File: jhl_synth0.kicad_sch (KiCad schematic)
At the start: 17 parts, among them J1 Conn_01x04, J2 USB_B_Micro, J3 Conn_01x04, J4 Conn_01x04, J5 Conn_01x01, J7 Conn_01x08, U1 YAAJ_BluePill, U2 YAAJ_BlackPill, U3 NUCLEO-F303K8

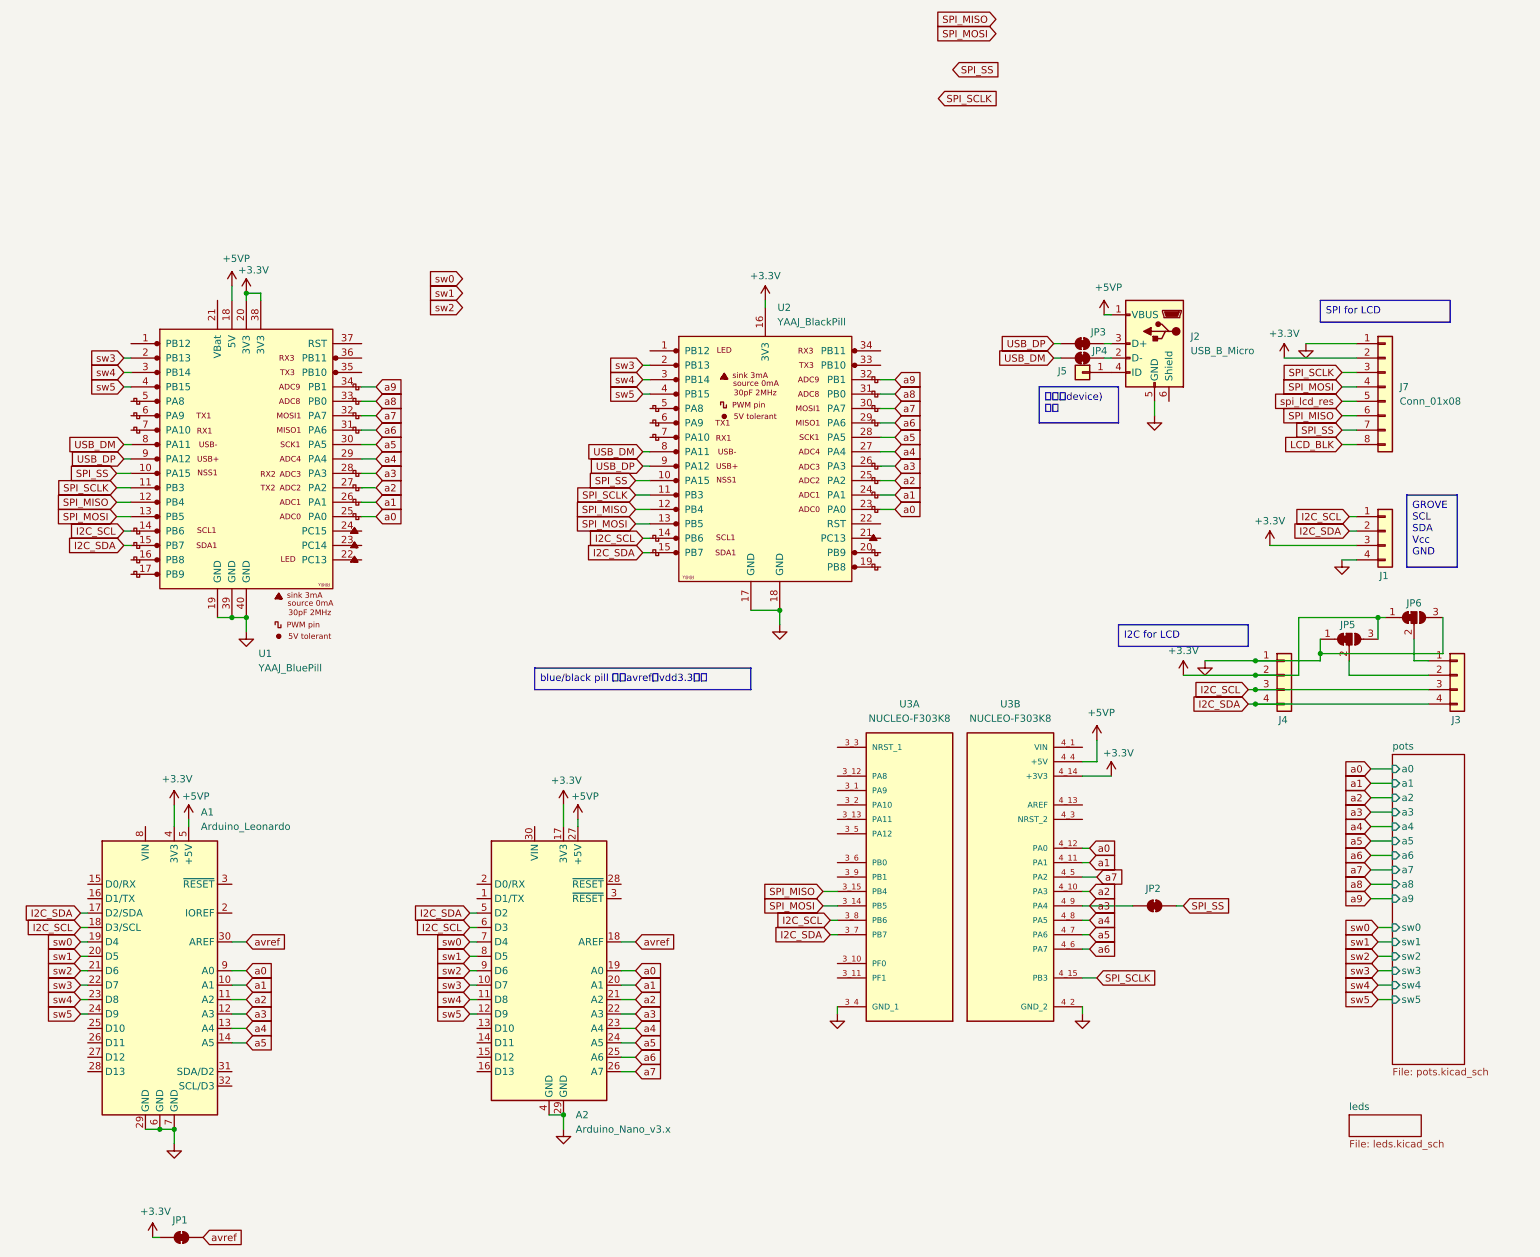
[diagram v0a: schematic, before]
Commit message: 251023
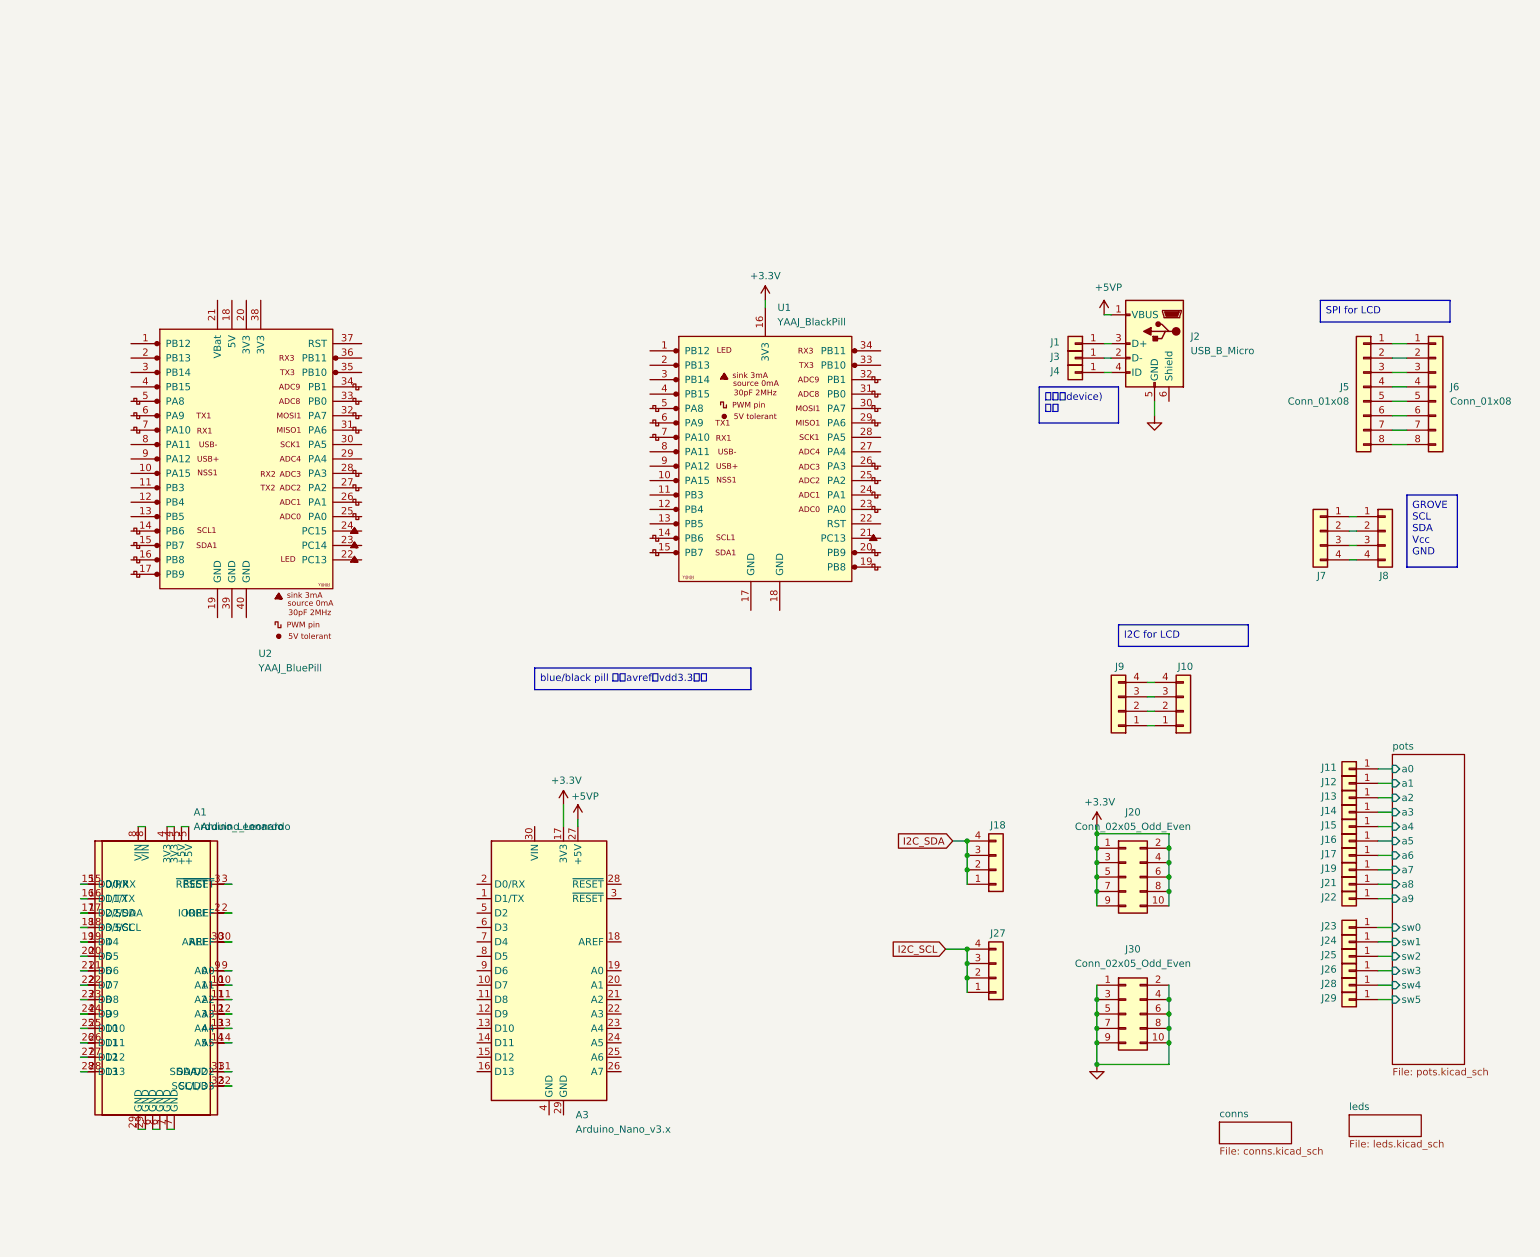
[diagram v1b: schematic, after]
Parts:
- removed J3, J4: Conn_01x04, Connector_PinSocket_2.54mm:PinSocket_1x04_P2.54mm_Vertical, symbol Connector_Generic:Conn_01x04
- removed JP1, JP2, JP3, JP4: SolderJumper_2_Bridged, Jumper:SolderJumper-2_P1.3mm_Bridged_RoundedPad1.0x1.5mm, symbol Jumper:SolderJumper_2_Bridged
- removed JP5, JP6: SolderJumper_3_Bridged12, Jumper:SolderJumper-3_P1.3mm_Bridged12_RoundedPad1.0x1.5mm, symbol Jumper:SolderJumper_3_Bridged12
- removed U3: NUCLEO-F303K8, NUCLEO-F303K8:MODULE_NUCLEO-F303K8, symbol NUCLEO-F303K8:NUCLEO-F303K8
- added A1: Arduino_Leonardo, Module:Arduino_UNO_R3, symbol MCU_Module:Arduino_Leonardo
- added J1, J11, J12, J13, J14, J15, J16, J17, J19, J21, J22, J23, J24, J25, J26, J28, J29, J3: Conn_01x01, Connector_PinSocket_2.54mm:PinSocket_1x01_P2.54mm_Vertical, symbol Connector_Generic:Conn_01x01
- added J10, J18, J27, J7, J9: Conn_01x04, Connector_PinSocket_2.54mm:PinSocket_1x04_P2.54mm_Vertical, symbol Connector_Generic:Conn_01x04
- added J20, J30: Conn_02x05_Odd_Even, Connector_PinHeader_2.54mm:PinHeader_2x05_P2.54mm_Vertical, symbol Connector_Generic:Conn_02x05_Odd_Even
- added J6: Conn_01x08, Connector_PinHeader_2.54mm:PinHeader_1x08_P2.54mm_Vertical, symbol Connector_Generic:Conn_01x08
- renumbered A1 to A2, A2 to A3, J5 to J4, J7 to J5, J1 to J8, U2 to U1, U1 to U2
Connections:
- net +3.3V: now also J20.1 (Pin_1), J20.10 (Pin_10), J20.2 (Pin_2), J20.3 (Pin_3), J20.4 (Pin_4), J20.5 (Pin_5), J20.6 (Pin_6), J20.7 (Pin_7), J20.8 (Pin_8), J20.9 (Pin_9); no longer A2.4 (3V3), J5.2 (Pin_2), J8.3 (Pin_3), U2.20 (3V3), U2.38 (3V3)
- net +5VP: no longer A2.5 (+5V), U2.18 (5V)
- net GND: now also J30.1 (Pin_1), J30.10 (Pin_10), J30.2 (Pin_2), J30.3 (Pin_3), J30.4 (Pin_4), J30.5 (Pin_5), J30.6 (Pin_6), J30.7 (Pin_7), J30.8 (Pin_8), J30.9 (Pin_9); no longer A2.29 (GND), A2.6 (GND), A2.7 (GND), A3.29 (GND), A3.4 (GND), J5.1 (Pin_1), J8.4 (Pin_4), U1.17 (GND), U1.18 (GND), U2.19 (GND), U2.39 (GND), U2.40 (GND)
- net I2C_SCL: now also J27.1 (Pin_1), J27.2 (Pin_2), J27.3 (Pin_3), J27.4 (Pin_4); no longer A2.18 (D3/SCL), A3.6 (D3), J8.1 (Pin_1), U1.14 (PB6), U2.14 (PB6)
- net I2C_SDA: now also J18.1 (Pin_1), J18.2 (Pin_2), J18.3 (Pin_3), J18.4 (Pin_4); no longer A2.17 (D2/SDA), A3.5 (D2), J8.2 (Pin_2), U1.15 (PB7), U2.15 (PB7)
- net at J2.2 (D-): now also J3.1 (Pin_1)
- net at J2.3 (D+): now also J1.1 (Pin_1)
- net at A2.15 (D0/RX): now also A1.15 (D0/RX)
- net at A2.16 (D1/TX): now also A1.16 (D1/TX)
- net at A2.2 (IOREF): now also A1.2 (IOREF)
- net at A2.25 (D10): now also A1.25 (D10)
- net at A2.26 (D11): now also A1.26 (D11)
- net at A2.27 (D12): now also A1.27 (D12)
- net at A2.28 (D13): now also A1.28 (D13)
- net at A2.3 (~{RESET}): now also A1.3 (~{RESET})
- net at A2.31 (SDA/D2): now also A1.31 (SDA/D2)
- net at A2.32 (SCL/D3): now also A1.32 (SCL/D3)
- net at A2.8 (VIN): now also A1.8 (VIN)
- net LCD_BLK: no longer names the net of J5.8 (Pin_8)
- net LCD_BLK: now also J6.8 (Pin_8)
- removed net SPI_MISO: J5.6 (Pin_6), U1.12 (PB4), U2.12 (PB4)
- removed net SPI_MOSI: J5.4 (Pin_4), U1.13 (PB5), U2.13 (PB5)
- removed net SPI_SCLK: J5.3 (Pin_3), U1.11 (PB3), U2.11 (PB3)
- removed net SPI_SS: J5.7 (Pin_7), U1.10 (PA15), U2.10 (PA15)
- net USB_DM: no longer names the net of U1.8 (PA11)
- net USB_DM: no longer U2.8 (PA11)
- net USB_DP: no longer names the net of U1.9 (PA12)
- net USB_DP: no longer U2.9 (PA12)
- removed net a0: A2.9 (A0), A3.19 (A0), U1.23 (PA0), U2.25 (PA0)
- removed net a1: A2.10 (A1), A3.20 (A1), U1.24 (PA1), U2.26 (PA1)
- removed net a2: A2.11 (A2), A3.21 (A2), U1.25 (PA2), U2.27 (PA2)
- removed net a3: A2.12 (A3), A3.22 (A3), U1.26 (PA3), U2.28 (PA3)
- removed net a4: A2.13 (A4), A3.23 (A4), U1.27 (PA4), U2.29 (PA4)
- removed net a5: A2.14 (A5), A3.24 (A5), U1.28 (PA5), U2.30 (PA5)
- removed net a6: A3.25 (A6), U1.29 (PA6), U2.31 (PA6)
- removed net a7: A3.26 (A7), U1.30 (PA7), U2.32 (PA7)
- net a8: no longer names the net of U1.31 (PB0)
- net a8: no longer U2.33 (PB0)
- net a9: no longer names the net of U1.32 (PB1)
- net a9: no longer U2.34 (PB1)
- net avref: no longer names the net of A3.18 (AREF)
- net avref: no longer A2.30 (AREF)
- net spi_lcd_res: no longer names the net of J5.5 (Pin_5)
- net spi_lcd_res: now also J6.5 (Pin_5)
- net sw0: no longer names the net of A3.7 (D4)
- net sw0: no longer A2.19 (D4)
- net sw1: no longer names the net of A3.8 (D5)
- net sw1: no longer A2.20 (D5)
- net sw2: no longer names the net of A3.9 (D6)
- net sw2: no longer A2.21 (D6)
- removed net sw3: A2.22 (D7), A3.10 (D7), U1.2 (PB13), U2.2 (PB13)
- removed net sw4: A2.23 (D8), A3.11 (D8), U1.3 (PB14), U2.3 (PB14)
- removed net sw5: A2.24 (D9), A3.12 (D9), U1.4 (PB15), U2.4 (PB15)
- new net: J7.1 (Pin_1), J8.1 (Pin_1)
- new net: J7.2 (Pin_2), J8.2 (Pin_2)
- new net: J7.3 (Pin_3), J8.3 (Pin_3)
- new net: J7.4 (Pin_4), J8.4 (Pin_4)
- new net: J5.1 (Pin_1), J6.1 (Pin_1)
- new net: J5.2 (Pin_2), J6.2 (Pin_2)
- new net: J5.3 (Pin_3), J6.3 (Pin_3)
- new net: J5.4 (Pin_4), J6.4 (Pin_4)
- new net: J5.6 (Pin_6), J6.6 (Pin_6)
- new net: J5.7 (Pin_7), J6.7 (Pin_7)
- new net: J10.1 (Pin_1), J9.1 (Pin_1)
- new net: J10.2 (Pin_2), J9.2 (Pin_2)
- new net: J10.3 (Pin_3), J9.3 (Pin_3)
- new net: J10.4 (Pin_4), J9.4 (Pin_4)
- new net: A1.10 (A1), A2.10 (A1)
- new net: A1.11 (A2), A2.11 (A2)
- new net: A1.12 (A3), A2.12 (A3)
- new net: A1.13 (A4), A2.13 (A4)
- new net: A1.14 (A5), A2.14 (A5)
- new net: A1.17 (D2/SDA), A2.17 (D2/SDA)
- new net: A1.18 (D3/SCL), A2.18 (D3/SCL)
- new net: A1.19 (D4), A2.19 (D4)
- new net: A1.20 (D5), A2.20 (D5)
- new net: A1.21 (D6), A2.21 (D6)
- new net: A1.22 (D7), A2.22 (D7)
- new net: A1.23 (D8), A2.23 (D8)
- new net: A1.24 (D9), A2.24 (D9)
- new net: A1.29 (GND), A2.29 (GND)
- new net: A1.30 (AREF), A2.30 (AREF)
- new net: A1.4 (3V3), A2.4 (3V3)
- new net: A1.5 (+5V), A2.5 (+5V)
- new net: A1.6 (GND), A2.6 (GND)
- new net: A1.7 (GND), A2.7 (GND)
- new net: A1.9 (A0), A2.9 (A0)
- new net pots/a0: J11.1 (Pin_1)
- new net pots/a1: J12.1 (Pin_1)
- new net pots/a2: J13.1 (Pin_1)
- new net pots/a3: J14.1 (Pin_1)
- new net pots/a4: J15.1 (Pin_1)
- new net pots/a5: J16.1 (Pin_1)
- new net pots/a6: J17.1 (Pin_1)
- new net pots/a7: J19.1 (Pin_1)
- new net pots/a8: J21.1 (Pin_1)
- new net pots/a9: J22.1 (Pin_1)
- new net pots/sw0: J23.1 (Pin_1)
- new net pots/sw1: J24.1 (Pin_1)
- new net pots/sw2: J25.1 (Pin_1)
- new net pots/sw3: J26.1 (Pin_1)
- new net pots/sw4: J28.1 (Pin_1)
- new net pots/sw5: J29.1 (Pin_1)
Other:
- added sheet conns (conns.kicad_sch)
- moved on the sheet: J4

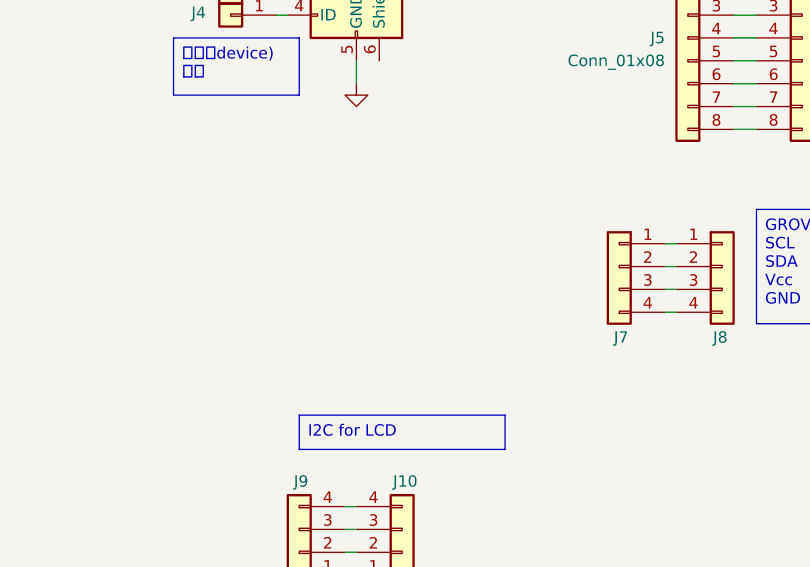
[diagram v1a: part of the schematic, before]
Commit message: 更新
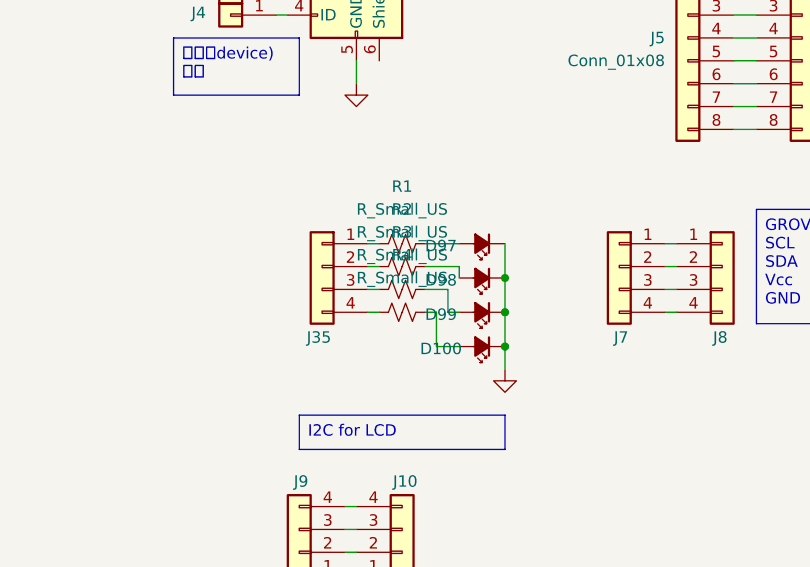
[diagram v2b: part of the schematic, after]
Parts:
- added D100, D97, D98, D99: LED_Small_Filled, LED_SMD:LED_0603_1608Metric_Pad1.05x0.95mm_HandSolder, symbol Device:LED_Small_Filled
- added J35: Conn_01x04, Connector_PinSocket_2.54mm:PinSocket_1x04_P2.54mm_Vertical, symbol Connector_Generic:Conn_01x04
- added R1, R2, R3, R4: R_Small_US, Resistor_SMD:R_0402_1005Metric_Pad0.72x0.64mm_HandSolder, symbol Device:R_Small_US
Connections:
- net GND: now also D100.1 (K), D97.1 (K), D98.1 (K), D99.1 (K)
- new net: J35.1 (Pin_1), R1.1
- new net: D97.2 (A), R1.2
- new net: J35.2 (Pin_2), R2.1
- new net: J35.3 (Pin_3), R3.1
- new net: J35.4 (Pin_4), R4.1
- new net: D98.2 (A), R2.2
- new net: D99.2 (A), R3.2
- new net: D100.2 (A), R4.2
